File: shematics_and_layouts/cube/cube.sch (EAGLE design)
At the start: 1 part

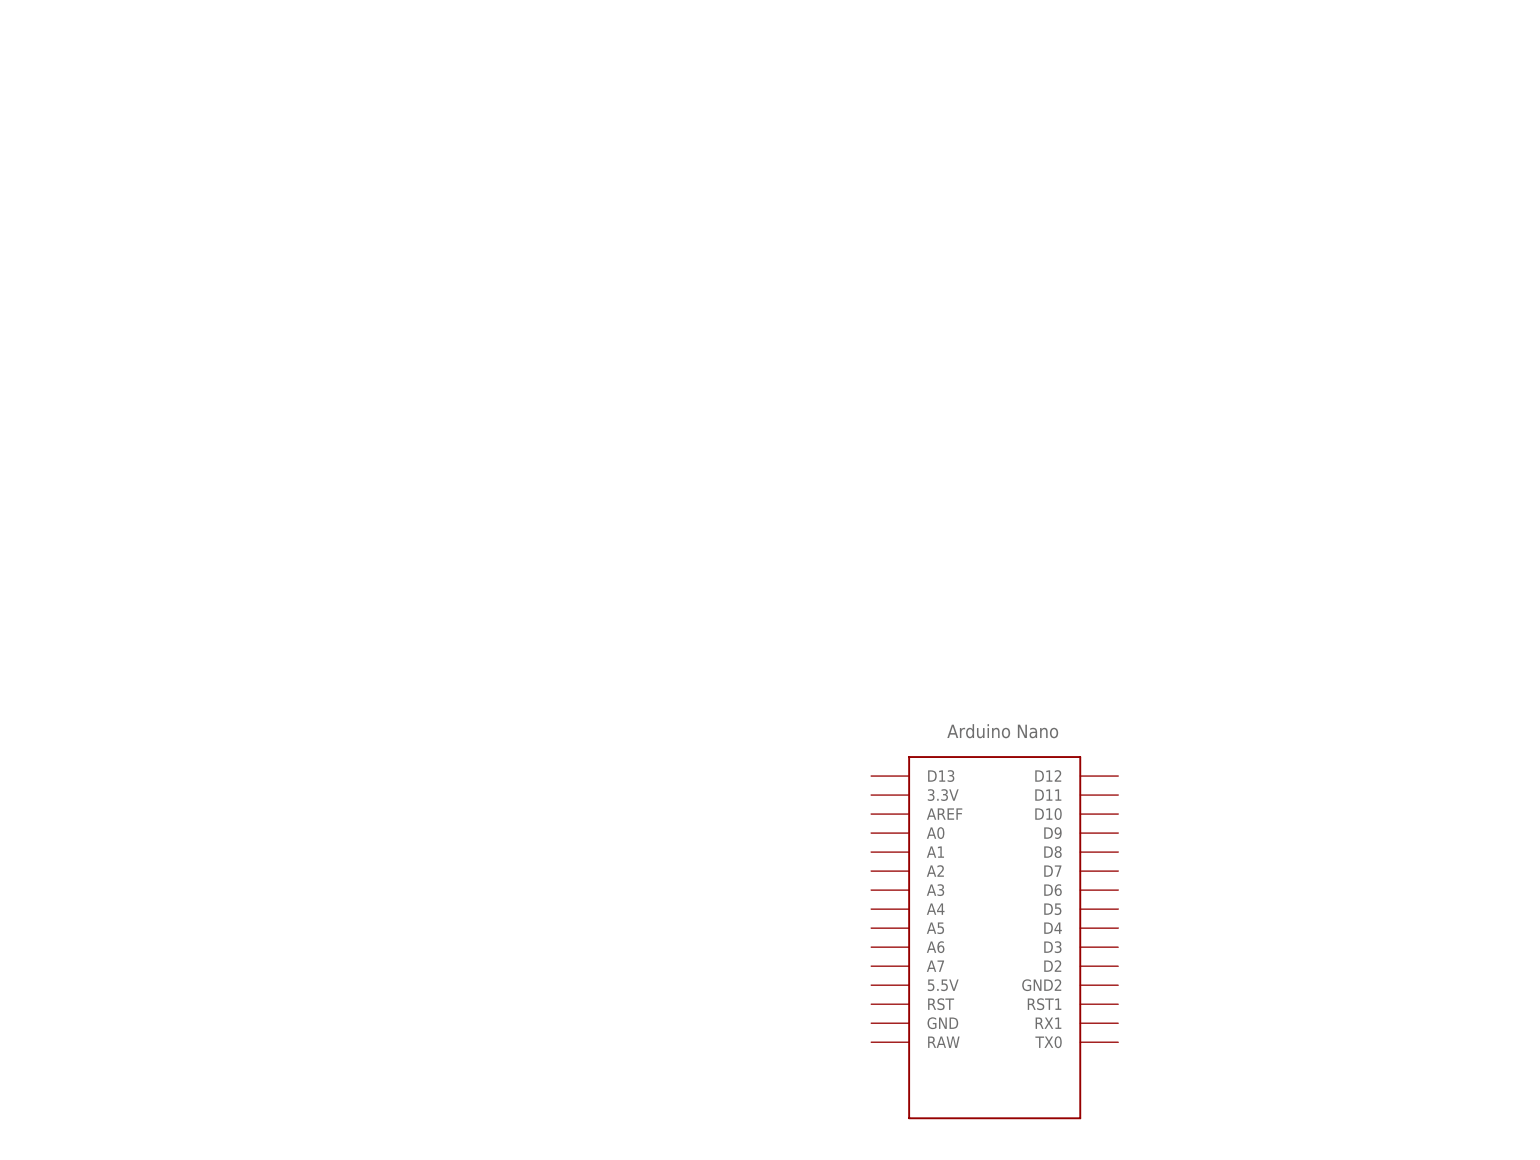
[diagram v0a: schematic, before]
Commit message: TASK: Basic and ugly cube shematic
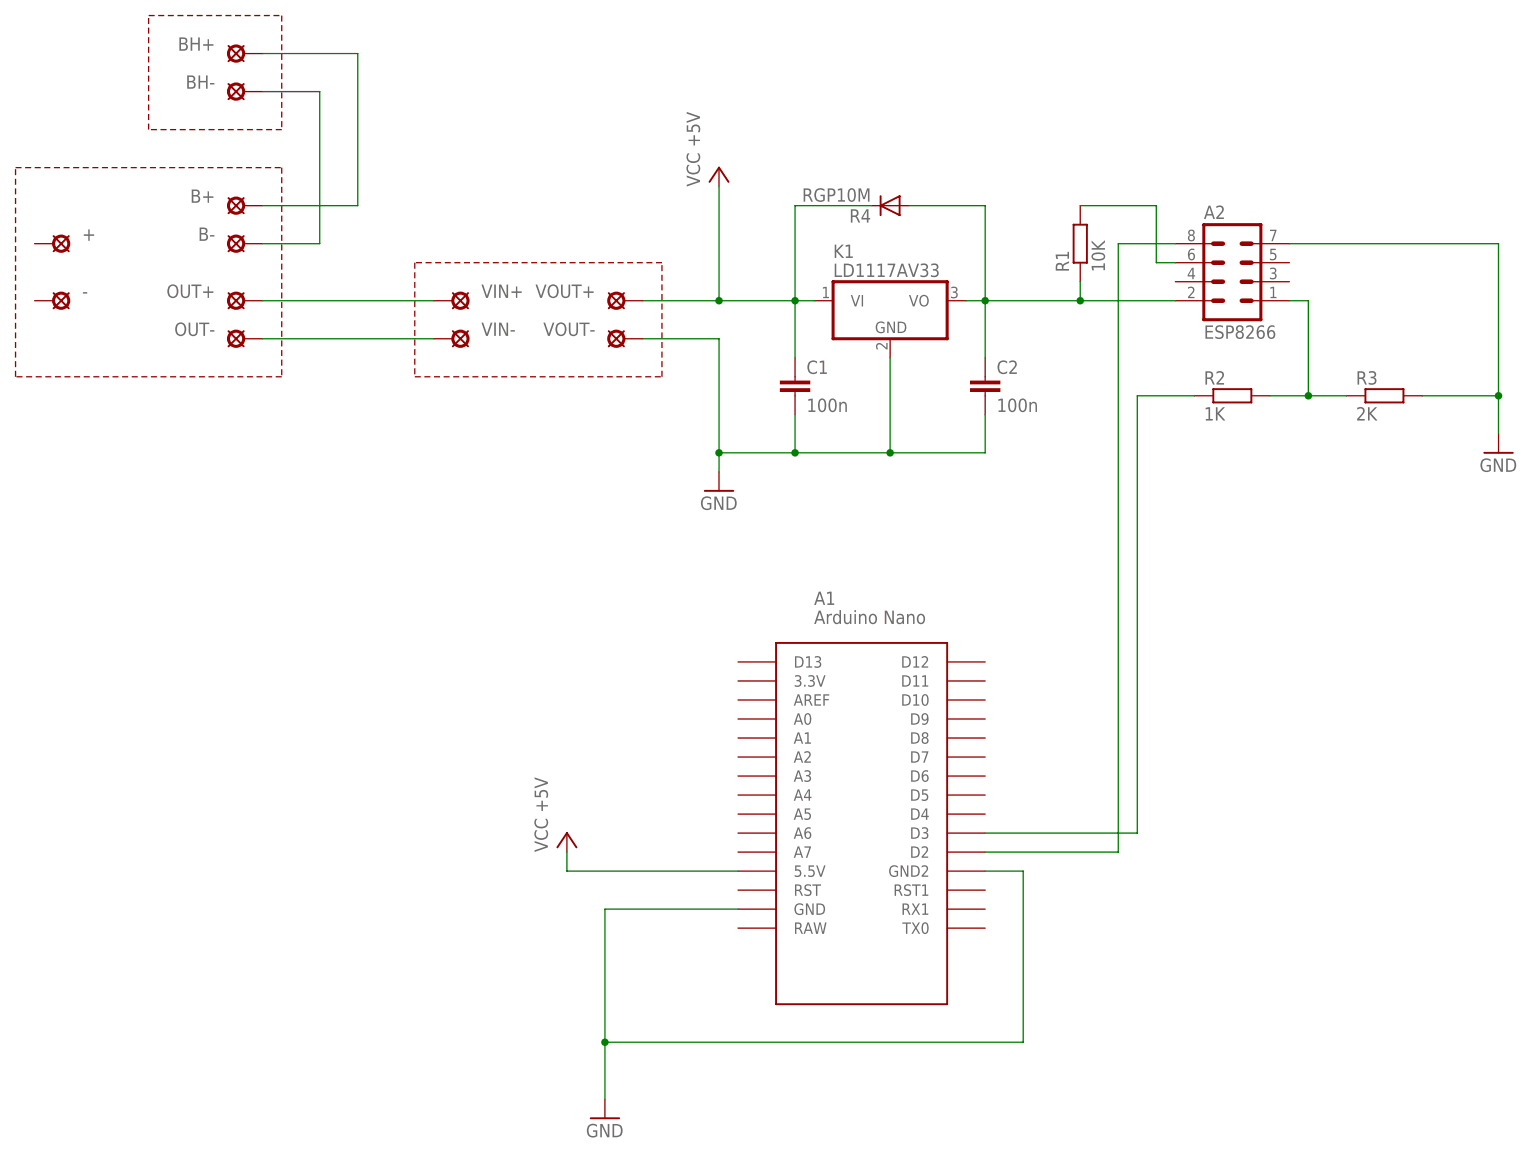
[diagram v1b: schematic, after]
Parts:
- added +, -, B+, B-, BH+, BH-, OUT+, OUT-, VIN+, VIN-, VOUT+, VOUT-: MCS08, solpad:MCS08
- added A2: ESP8266, con-lstb:MA04-2
- added C1, C2: 100n, rcl:C-EU050-024X044
- added K1: LD1117AV33, linear:7805T
- added R1: 10K, rcl:R-EU_0207/10
- added R2: 1K, rcl:R-EU_0207/10
- added R3: 2K, rcl:R-EU_0207/10
- added R4: RGP10M, diode:1N4446
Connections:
- new net GND: A1.GND, A1.GND2, A2.7, C1.2, C2.2, K1.GND, R3.2, VOUT-.MP
- new net N$1: OUT+.MP, VIN+.MP
- new net N$2: OUT-.MP, VIN-.MP
- new net N$3: A2.2, C2.1, K1.VO, R1.1, R4.A
- new net N$4: A2.1, R2.2, R3.1
- new net N$5: A2.6, R1.2
- new net N$6: A1.D2, A2.8
- new net N$7: B-.MP, BH-.MP
- new net N$8: A1.D3, R2.1
- new net N$9: B+.MP, BH+.MP
- new net VCC: A1.5.5V, C1.1, K1.VI, R4.C, VOUT+.MP
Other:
- note added: "A1"
